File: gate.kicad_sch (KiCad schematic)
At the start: 3 parts, among them U1 LM5113SD/NOPB, U2 LM5113SD/NOPB, U6 LM5113SD/NOPB

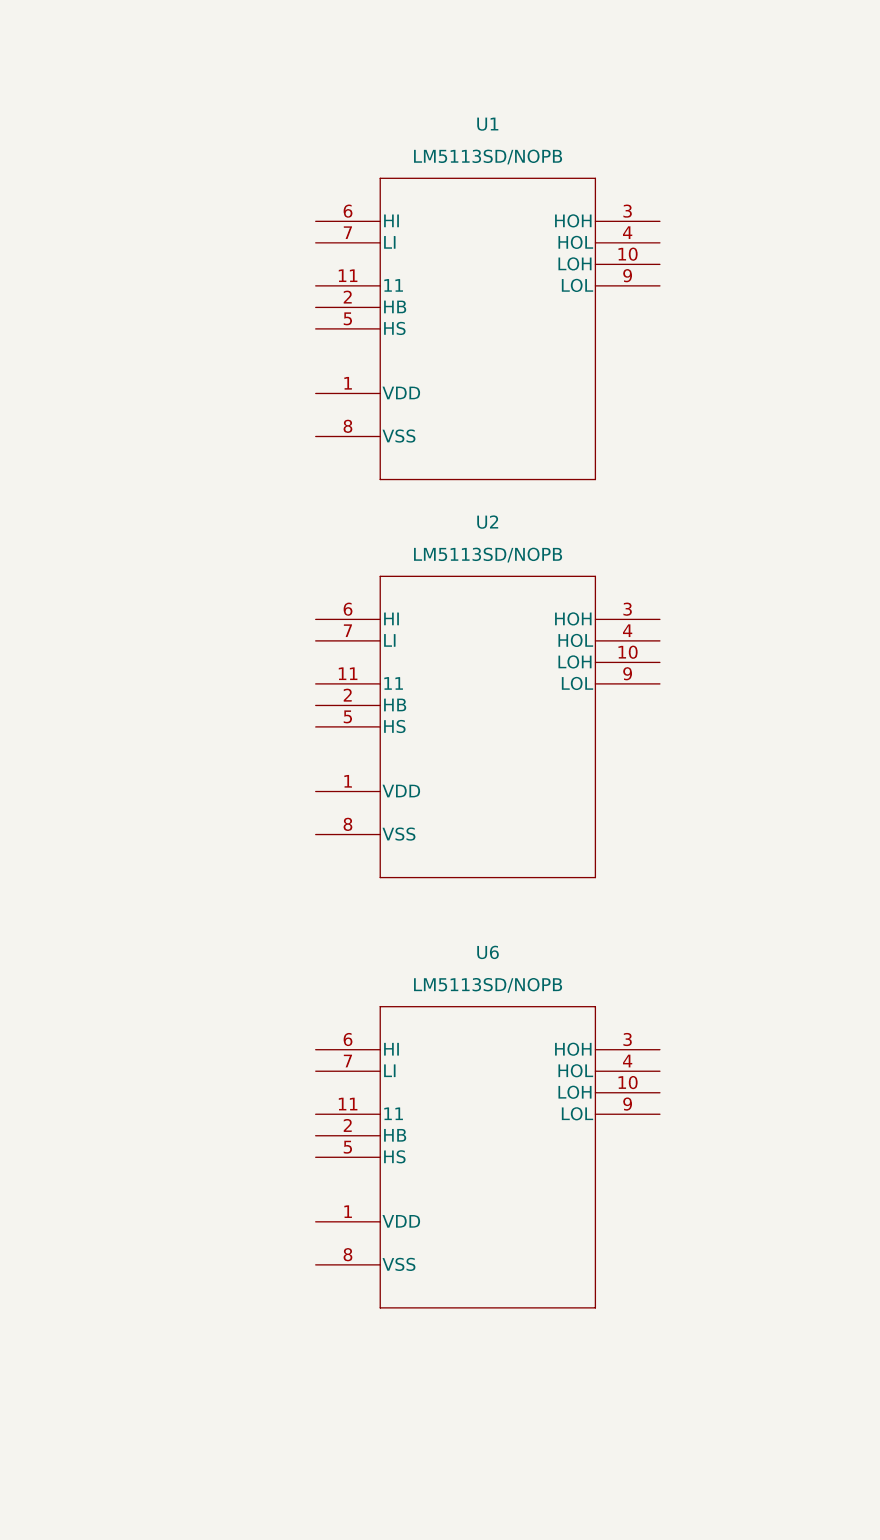
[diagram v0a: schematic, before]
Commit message: before changing connector
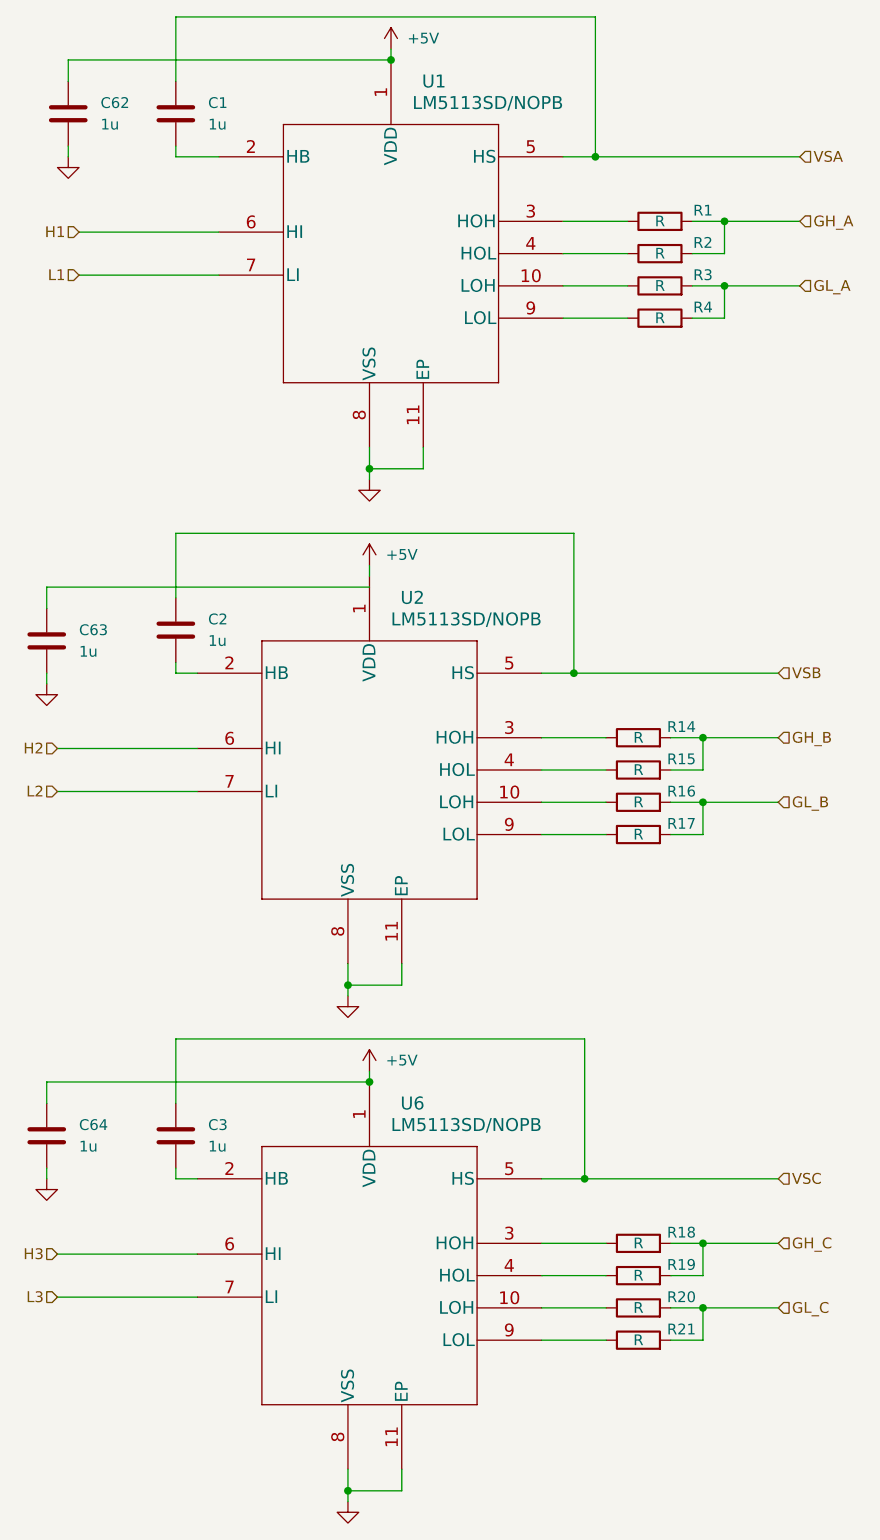
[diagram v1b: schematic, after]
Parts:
- added C1, C62, C63, C64: 1u, Capacitor_SMD:C_0402_1005Metric, symbol Device:C
- added C2, C3: 1u, Capacitor_SMD:C_0805_2012Metric, symbol Device:C
- added R1, R14, R15, R16, R17, R18, R19, R2, R20, R21, R3, R4: R, Resistor_SMD:R_0402_1005Metric, symbol Device:R
- U1, U2, U6: footprint lm5113:LM5113SD&slash_NOPB -> lm5113:LM5113SD_NOPB
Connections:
- net +5V: now reaches U1.1 (VDD)
- net +5V: now also U2.1 (VDD), U6.1 (VDD), C62.1, C64.1
- net at U1.10 (LOH): now also R3.1
- net GND: now reaches U1.11 (EP)
- net GND: now also U1.8 (VSS), U2.11 (EP), U2.8 (VSS), U6.11 (EP), U6.8 (VSS), C62.2, C63.2, C64.2
- net at U1.2 (HB): now also C1.2
- net at U1.3 (HOH): now also R1.1
- net at U1.4 (HOL): now also R2.1
- net VSA: now reaches U1.5 (HS)
- net VSA: now also C1.1
- net H1: now reaches U1.6 (HI)
- net L1: now reaches U1.7 (LI)
- net at U1.9 (LOL): now also R4.1
- net at U6.10 (LOH): now also R20.1
- net at U6.2 (HB): now also C3.2
- net at U6.3 (HOH): now also R18.1
- net at U6.4 (HOL): now also R19.1
- net VSC: now reaches U6.5 (HS)
- net VSC: now also C3.1
- net H3: now reaches U6.6 (HI)
- net L3: now reaches U6.7 (LI)
- net at U6.9 (LOL): now also R21.1
- net at U2.10 (LOH): now also R16.1
- net at U2.2 (HB): now also C2.2
- net at U2.3 (HOH): now also R14.1
- net at U2.4 (HOL): now also R15.1
- net VSB: now reaches U2.5 (HS)
- net VSB: now also C2.1
- net H2: now reaches U2.6 (HI)
- net L2: now reaches U2.7 (LI)
- net at U2.9 (LOL): now also R17.1
- new net GH_A: R1.2, R2.2
- new net GH_B: R14.2, R15.2
- new net GH_C: R18.2, R19.2
- new net GL_A: R3.2, R4.2
- new net GL_B: R16.2, R17.2
- new net GL_C: R20.2, R21.2
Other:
- moved on the sheet: U1

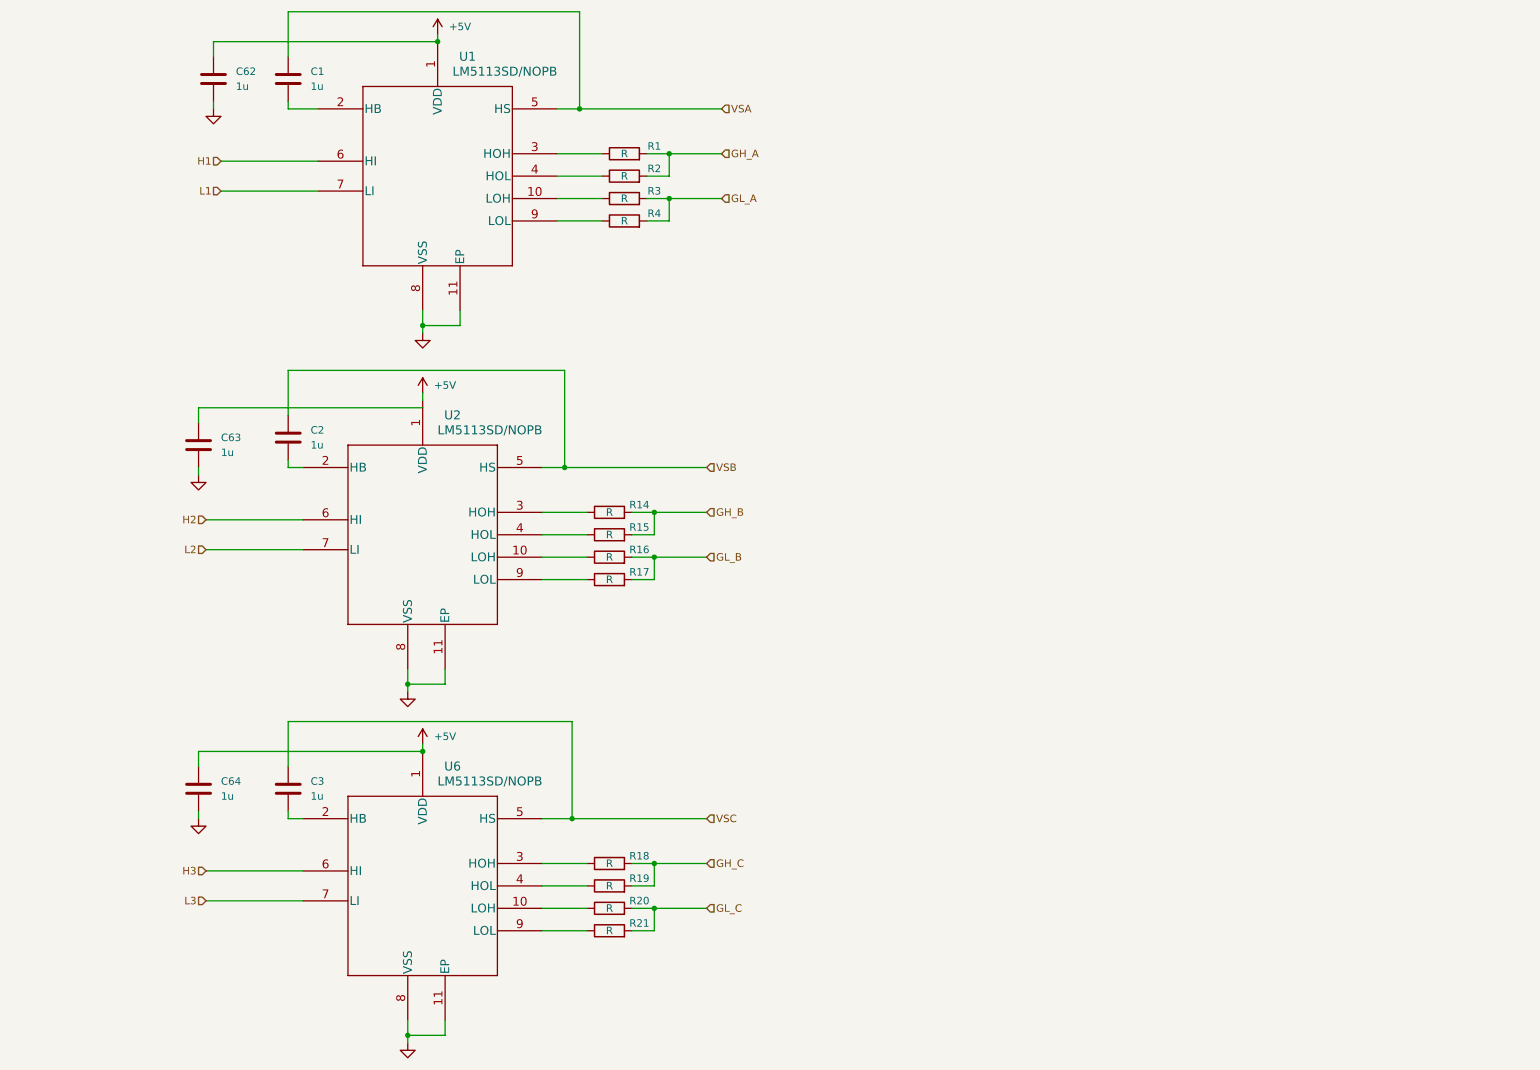
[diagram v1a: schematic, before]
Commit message: v0.1
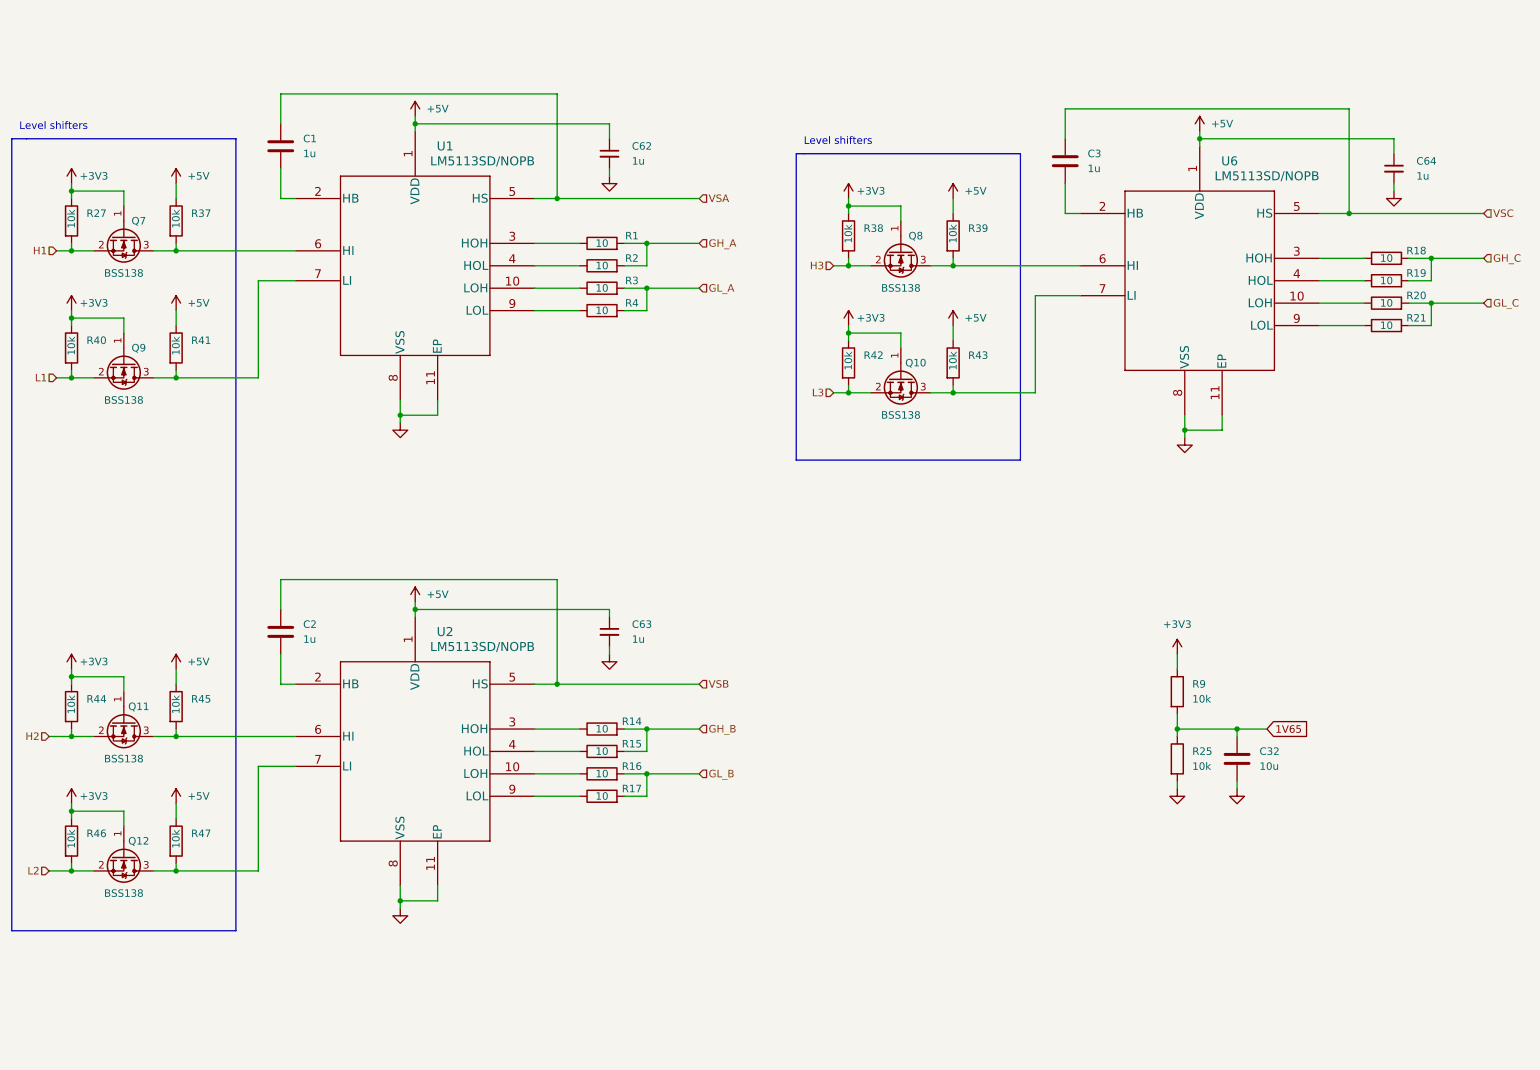
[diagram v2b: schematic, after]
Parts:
- added C32: 10u, Capacitor_SMD:C_0805_2012Metric, symbol Device:C
- added Q10, Q11, Q12, Q7, Q8, Q9: BSS138, Package_TO_SOT_SMD:SOT-23, symbol Transistor_FET:BSS138
- added R25, R27, R37, R38, R39, R40, R41, R42, R43, R44, R45, R46, R47, R9: 10k, Resistor_SMD:R_0805_2012Metric, symbol Device:R
- C1: footprint Capacitor_SMD:C_0402_1005Metric -> Capacitor_SMD:C_0805_2012Metric; LCSC (none) -> C319195
- C2, C3: LCSC (none) -> C319195
- C62, C63, C64: footprint Capacitor_SMD:C_0402_1005Metric -> Capacitor_SMD:C_0603_1608Metric; symbol Device:C -> Device:C_Small; LCSC (none) -> C319195
- R1, R2, R3, R4: value R -> 10; footprint Resistor_SMD:R_0402_1005Metric -> Resistor_SMD:R_0603_1608Metric; LCSC (none) -> C22859
- R14, R15, R16, R17: value R -> 10; footprint Resistor_SMD:R_0402_1005Metric -> Resistor_SMD:R_0603_1608Metric; LCSC (none) -> C23164
- R18, R19: value R -> 10; footprint Resistor_SMD:R_0402_1005Metric -> Resistor_SMD:R_0603_1608Metric; LCSC (none) -> C112307
- R20, R21: value R -> 10; footprint Resistor_SMD:R_0402_1005Metric -> Resistor_SMD:R_0603_1608Metric; LCSC (none) -> C2907056
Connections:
- net +5V: now also C63.1, R37.1, R39.1, R41.1, R43.1, R45.1, R47.1
- net GND: now also C32.2, R25.2
- net H1: now also Q7.2 (S), R27.2; no longer U1.6 (HI)
- net H2: now also Q11.2 (S), R44.2; no longer U2.6 (HI)
- net H3: now also Q8.2 (S), R38.2; no longer U6.6 (HI)
- net L1: now also Q9.2 (S), R40.2; no longer U1.7 (LI)
- net L2: now also Q12.2 (S), R46.2; no longer U2.7 (LI)
- net L3: now also Q10.2 (S), R42.2; no longer U6.7 (LI)
- new net: Q11.3 (D), R45.2, U2.6 (HI)
- new net: Q7.3 (D), R37.2, U1.6 (HI)
- new net: Q9.3 (D), R41.2, U1.7 (LI)
- new net: Q8.3 (D), R39.2, U6.6 (HI)
- new net: Q10.3 (D), R43.2, U6.7 (LI)
- new net: Q12.3 (D), R47.2, U2.7 (LI)
- new net +3V3: Q10.1 (G), Q11.1 (G), Q12.1 (G), Q7.1 (G), Q8.1 (G), Q9.1 (G), R27.1, R38.1, R40.1, R42.1, R44.1, R46.1, R9.1
- new net 1V65: C32.1, R25.1, R9.2
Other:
- note added: "Level shifters"
- moved on the sheet: C1, C2, C3, C62, C63, C64, R1, R14, R15, R16, R17, R18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
